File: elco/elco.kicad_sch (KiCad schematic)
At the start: 18 parts, among them J2 Motor / Power, J3 IO, J4 Barrel_Jack_MountingPin, SW1 SW_DPDT_x2, U1 TPSM53602RDA

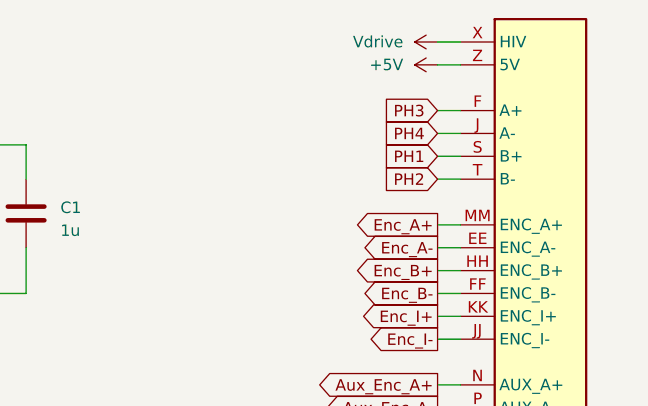
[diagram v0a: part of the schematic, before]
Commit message: Getting ready for fab
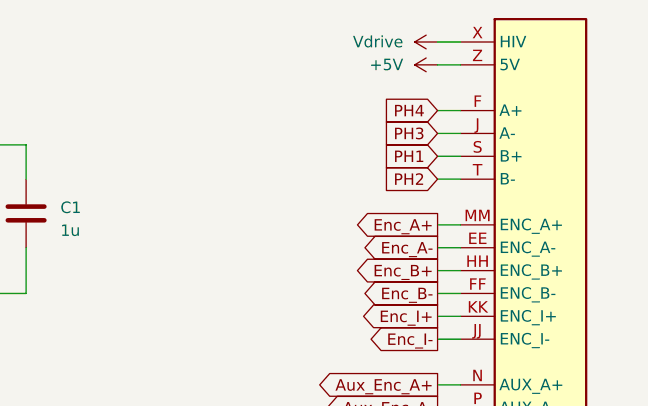
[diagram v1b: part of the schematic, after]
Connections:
- net PH3: now also J1.J (A-); no longer J1.F (A+)
- net PH4: now also J1.F (A+); no longer J1.J (A-)
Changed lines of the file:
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@@
     )
   )
-  (global_label "PH4" (shape input) (at 195.58 41.91 180) (fields_autoplaced)
+  (global_label "PH4" (shape input) (at 195.58 39.37 180) (fields_autoplaced)
     (effects (font (size 1.27 1.27)) (justify right))
-    (property "Intersheetrefs" "${INTERSHEET_REFS}" (at 188.8642 41.91 0)
+    (property "Intersheetrefs" "${INTERSHEET_REFS}" (at 188.8642 39.37 0)
       (effects (font (size 1.27 1.27)) (justify right) hide)
     )
@@
     )
   )
-  (global_label "PH3" (shape input) (at 195.58 39.37 180) (fields_autoplaced)
+  (global_label "PH3" (shape input) (at 195.58 41.91 180) (fields_autoplaced)
     (effects (font (size 1.27 1.27)) (justify right))
-    (property "Intersheetrefs" "${INTERSHEET_REFS}" (at 188.8642 39.37 0)
+    (property "Intersheetrefs" "${INTERSHEET_REFS}" (at 188.8642 41.91 0)
       (effects (font (size 1.27 1.27)) (justify right) hide)
     )
